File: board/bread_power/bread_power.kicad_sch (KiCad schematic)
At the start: 11 parts, among them J1 USB_C_Receptacle_PowerOnly_6P, U1 TPS61022, U2 BQ24073RGT

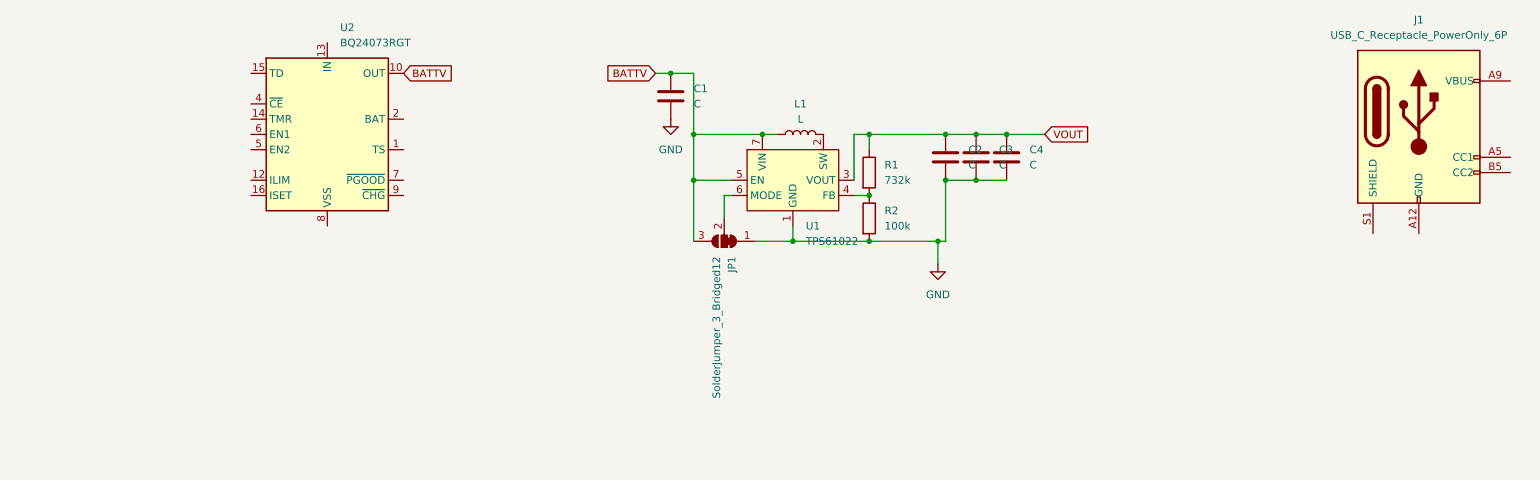
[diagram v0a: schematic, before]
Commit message: Adding some layout for the BMS circuit.
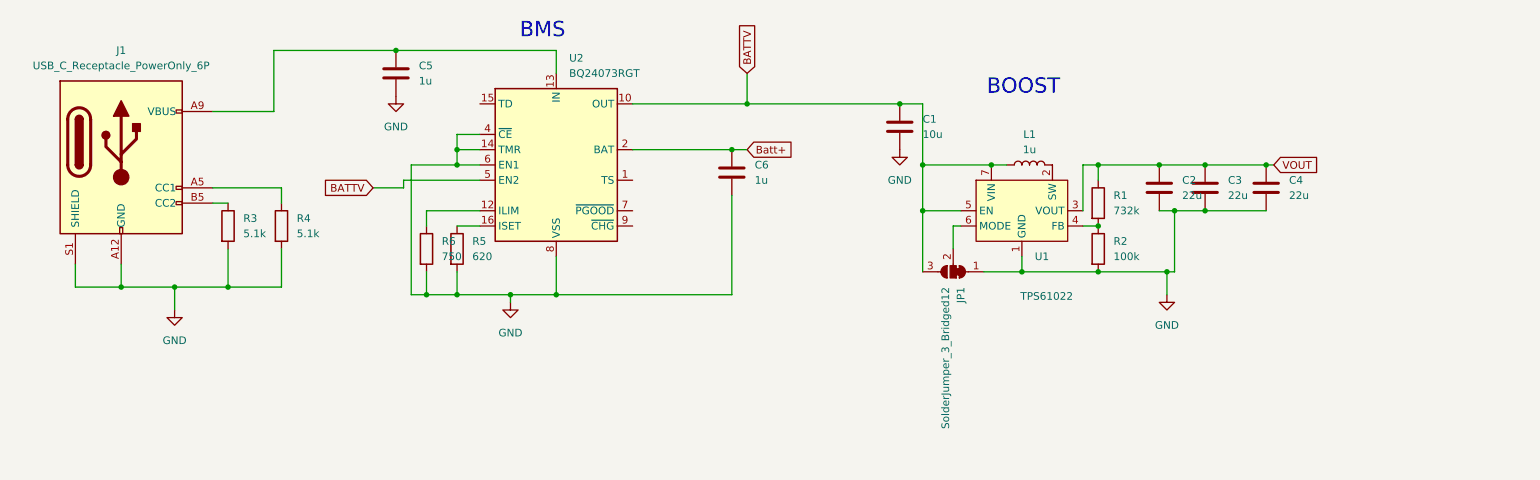
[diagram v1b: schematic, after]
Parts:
- added C5, C6: 1u, symbol Device:C
- added R3, R4: 5.1k, symbol Device:R
- added R5: 620, symbol Device:R
- added R6: 750, symbol Device:R
- C1: value C -> 10u
- C2, C3, C4: value C -> 22u
- L1: value L -> 1u
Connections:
- net BATTV: now also U2.5 (EN2)
- net GND: now also J1.A12 (GND), J1.B12 (GND), J1.S1 (SHIELD), U2.14 (TMR), U2.17 (VSS), U2.4 (~{CE}), U2.6 (EN1), U2.8 (VSS), C5.2, C6.2, R3.2, R4.2, R5.2, R6.2
- net at J1.A5 (CC1): now also R4.1
- net at J1.A9 (VBUS), J1.B9 (VBUS): now also U2.13 (IN), C5.1
- net at J1.B5 (CC2): now also R3.1
- net at U2.12 (ILIM): now also R6.1
- net at U2.16 (ISET): now also R5.1
- net Batt+: now reaches U2.2 (BAT), U2.3 (BAT)
- net Batt+: now also C6.1
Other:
- note added: "BMS"
- note added: "BOOST"
- moved on the sheet: C1, C2, C3, C4, J1, JP1, L1, R1, R2, U1, U2
